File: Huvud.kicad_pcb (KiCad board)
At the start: 4 copper layers, 42 x 42 mm, 109 parts, among them J1 TMC2209_BIGTREETECH_V1.2_HEAD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, J10 Probe, J11 TMC2209_BIGTREETECH_V1.2_HEAD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, J12 5V, J2 DBG, J3 THERM, J4 FAN0, J5 FAN1, J6 Heater, J7 Endstop, J8 TMC2209_BIGTREETECH_V1.2_HEAD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, J9 STEPPER, Q1 AO3400A, Q2 AO3400A, Q3 AON7524, U1 ADXL345, U3 TPS54202, U4 XC6206PxxxMR, U5 STM32F103C8T6, U6 TMC2209_BIGTREETECH_V1.2_MODU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, U7 HUSB238, Y1 8Mhz

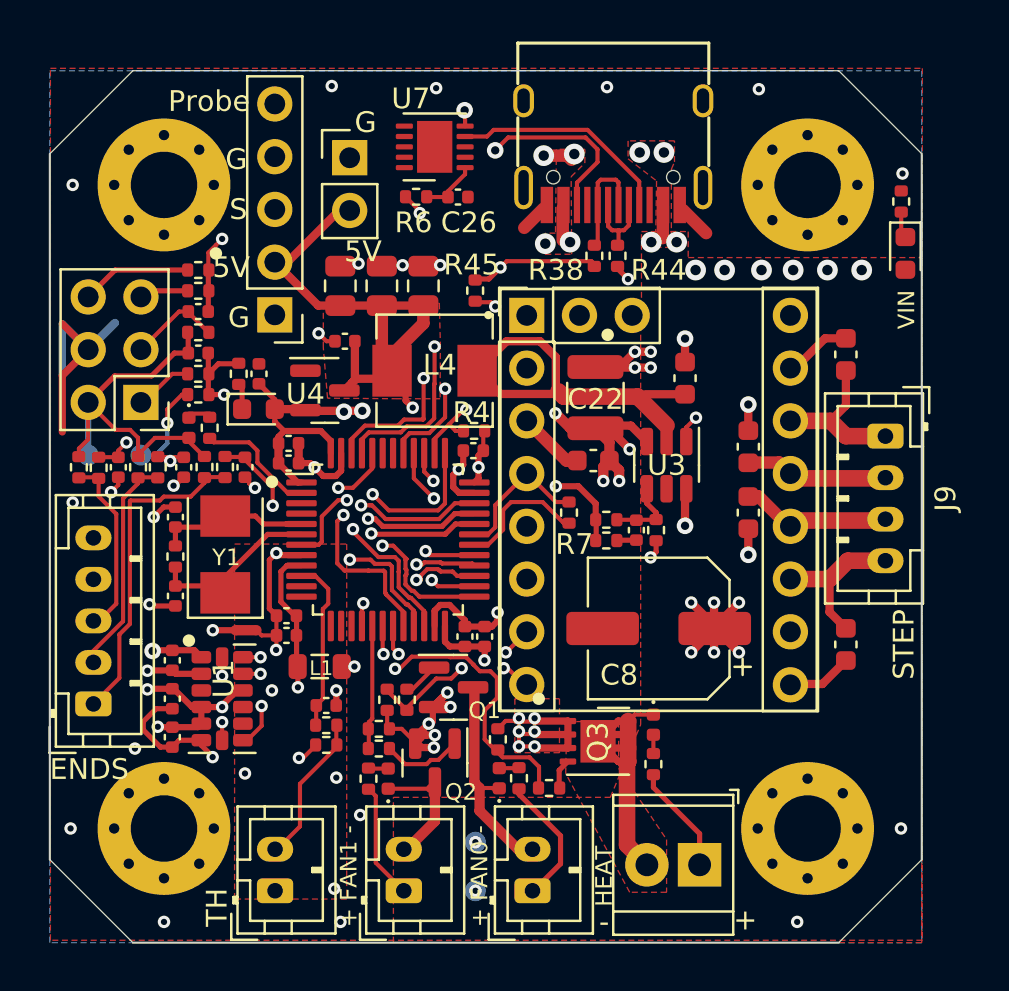
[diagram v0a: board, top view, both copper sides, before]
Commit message: cleanup and bom
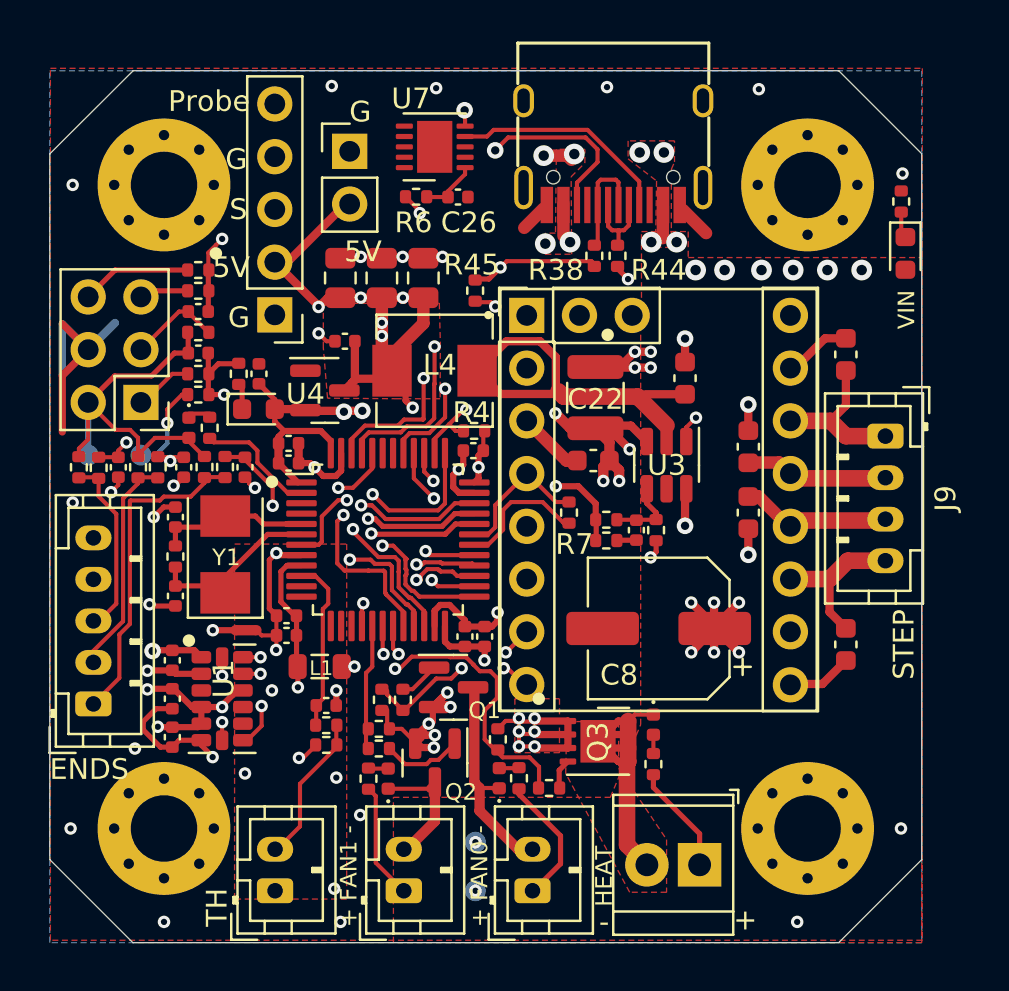
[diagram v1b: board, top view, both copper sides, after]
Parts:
- moved C14 0.38 mm to (200.0, 110.0)
- moved C15 0.38 mm to (196.0, 110.0)
- moved C32 0.38 mm to (198.0, 110.0)
- moved J12 0.31 mm to (196.4, 103.9)
- moved R8 0.26 mm to (198.0, 130.3)
- moved R34 0.19 mm to (199.0, 130.3)
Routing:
- net +5V: track 39.2 -> 36.2 mm, vias 2 -> 7
- net GND: track 101.9 -> 99.4 mm
- net Net-(U5-PD1): track 9.29 -> 7.41 mm
- net +3V3: track 116.8 -> 115.3 mm
- net ST_A1: track 12.2 -> 10.8 mm
- net ST_VS: track 52.6 -> 51.6 mm
- net Net-(D3-K): track 15.6 -> 14.6 mm
- net Net-(U5-PD0): track 8.08 -> 7.32 mm
- net BOOT1: track 23.0 -> 22.4 mm
- net ST_B1: track 12.1 -> 11.5 mm
